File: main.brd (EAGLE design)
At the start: 78.8 x 63 mm, 8 parts, among them X1 FH12-40S-0.5SH

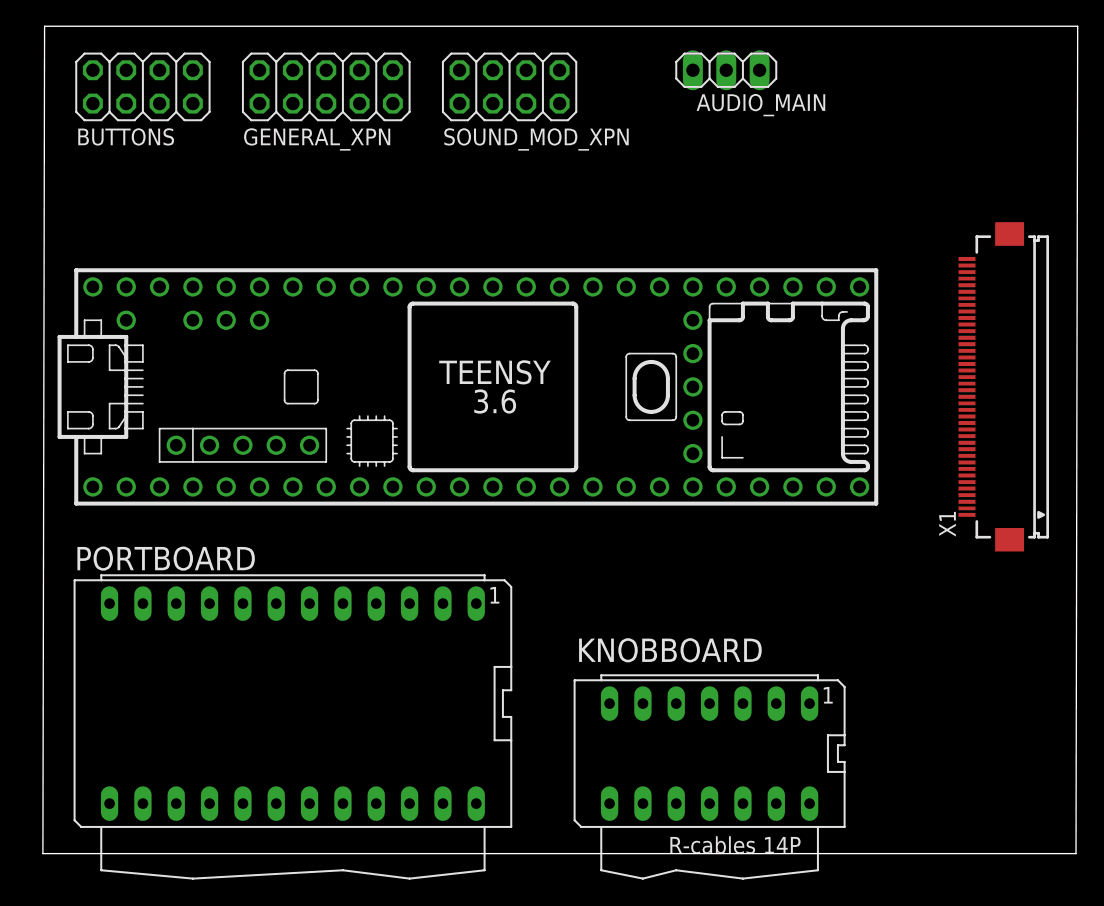
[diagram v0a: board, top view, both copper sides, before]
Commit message: Milestone fully drafted
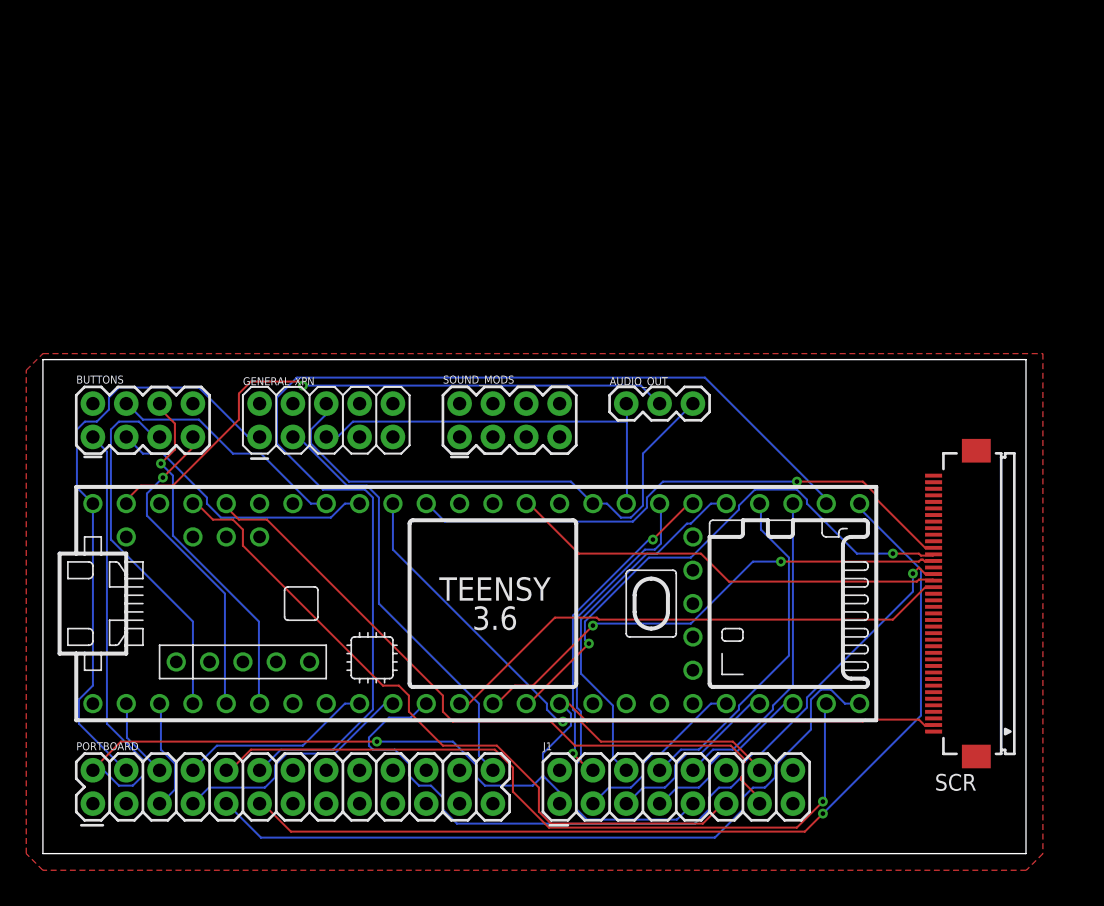
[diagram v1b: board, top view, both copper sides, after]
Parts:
- removed AUDIO_MAIN: (no value), pinhead:1X03
- removed KNOBBOARD: (no value), con-dil:IC14PL
- removed SOUND_MOD_XPN: (no value), pinhead:2X04
- removed X1: FH12-40S-0.5SH, con-hirose:FH12-40S-0.5SH
- added AUDIO_OUT: (no value), SparkFun-Connectors:1X03
- added J1: (no value), SparkFun-Connectors:2X8
- added SCR: FH12-40S-0.5SH, con-hirose:FH12-40S-0.5SH
- added SOUND_MODS: (no value), SparkFun-Connectors:2X4
- BUTTONS: device pinhead:2X04 -> SparkFun-Connectors:2X4
- GENERAL_XPN: device pinhead:2X05 -> SparkFun-Connectors:2X5
- PORTBOARD: device con-dil:IC24PL -> SparkFun-Connectors:2X13
- moved GENERAL_XPN 27.1 mm to (16.5, 31.8)
- moved BUTTONS 25.4 mm to (7.62, 33.0)
- moved PORTBOARD 17.0 mm to (3.81, 3.81), turned to 0 degrees
- moved U$1 16.5 mm to (31.8, 19.1)
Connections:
- removed net N$13: U$1.28
- removed net N$14: U$1.29
- removed net N$15: U$1.30
- removed net N$18: U$1.23/A9
- removed net N$19: U$1.22/A8
- removed net N$24: U$1.17/A3
- removed net N$30: U$1.35/A16
- removed net N$31: U$1.36/A17
- removed net N$32: U$1.37/A18
- removed net N$33: U$1.38/A19
- removed net N$34: U$1.39/A20
- new net USBDATA+: PORTBOARD.13
- new net USBDATA-: PORTBOARD.14
- net +12V: now also PORTBOARD.26
- net +3V3: now also J1.1, PORTBOARD.2, SCR.2; no longer KNOBBOARD.1, PORTBOARD.24, X1.2
- net +5V: now also PORTBOARD.4; no longer PORTBOARD.23
- net AUDIO_GND: now also AUDIO_OUT.2; no longer AUDIO_MAIN.2
- net AUDIO_L: now also AUDIO_OUT.1; no longer AUDIO_MAIN.1
- net AUDIO_R: now also AUDIO_OUT.3; no longer AUDIO_MAIN.3
- net GND: now also J1.2, PORTBOARD.3, SCR.1; no longer KNOBBOARD.14, PORTBOARD.2, X1.1
- net JOYSTICK_B: now also J1.14, U$1.17/A3; no longer KNOBBOARD.8
- net JOYSTICK_X: now also J1.11, U$1.23/A9; no longer KNOBBOARD.6
- net JOYSTICK_Y: now also J1.13, U$1.22/A8; no longer KNOBBOARD.7
- net MIDIIN1: now also PORTBOARD.6; no longer PORTBOARD.22
- net MIDIIN2: now also PORTBOARD.8; no longer PORTBOARD.21
- net MIDIIN3: now also PORTBOARD.10; no longer PORTBOARD.20
- net MIDIIN4: now also PORTBOARD.12; no longer PORTBOARD.19
- net MIDIOUT1: now also PORTBOARD.5; no longer PORTBOARD.3
- net MIDIOUT2: now also PORTBOARD.7; no longer PORTBOARD.4
- net MIDIOUT3: now also PORTBOARD.9; no longer PORTBOARD.5
- net MIDIOUT4: now also PORTBOARD.11; no longer PORTBOARD.6
- net ROTENC1_A: now also J1.3, U$1.28; no longer KNOBBOARD.2
- net ROTENC1_B: now also J1.5, U$1.29; no longer KNOBBOARD.3
- net ROTENC2_A: now also J1.7, U$1.30; no longer KNOBBOARD.4
- net ROTENC2_B: now also J1.9, U$1.39/A20; no longer KNOBBOARD.5
- net ROTENC3_A: now also J1.4, U$1.38/A19; no longer KNOBBOARD.13
- net ROTENC3_B: now also J1.6, U$1.37/A18; no longer KNOBBOARD.12
- net ROTENC4_A: now also J1.8, U$1.36/A17; no longer KNOBBOARD.11
- net ROTENC4_B: now also J1.10, U$1.35/A16; no longer KNOBBOARD.10
- net SCR_BL: now also SCR.29; no longer X1.29
- net SCR_CLK: now also SCR.24; no longer X1.24
- net SCR_CS: now also SCR.23; no longer X1.23
- net SCR_DC: now also SCR.25; no longer X1.25
- net SCR_MOSI: now also SCR.27; no longer X1.27
- net SCR_MOSO: now also SCR.28; no longer X1.28
- net SDCLK: now also PORTBOARD.19; no longer PORTBOARD.9
- net SDCMD: now also PORTBOARD.20; no longer PORTBOARD.16
- net SDDATA0: now also PORTBOARD.15; no longer PORTBOARD.7
- net SDDATA1: now also PORTBOARD.16; no longer PORTBOARD.18
- net SDDATA2: now also PORTBOARD.17; no longer PORTBOARD.8
- net SDDATA3: now also PORTBOARD.18; no longer PORTBOARD.17
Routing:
- net +3V3: track 0.00 -> 108.3 mm, vias 0 -> 1
- net MIDIIN4: track 0.00 -> 86.0 mm
- net MIDIOUT4: track 0.00 -> 73.1 mm, vias 0 -> 1
- net SCR_DC: track 0.00 -> 63.2 mm, vias 0 -> 1
- net MIDIIN3: track 0.00 -> 58.1 mm, vias 0 -> 1
- net MIDIOUT3: track 0.00 -> 56.9 mm
- net JOYSTICK_X: track 0.00 -> 53.9 mm
- net JOYSTICK_Y: track 0.00 -> 52.6 mm
- net AUDIO_GND: track 0.00 -> 46.5 mm, vias 0 -> 1
- net +5V: track 0.00 -> 45.8 mm
- net SCR_BL: track 0.00 -> 43.2 mm, vias 0 -> 1
- net SCR_MOSO: track 0.00 -> 41.7 mm, vias 0 -> 2
- net AUDIO_R: track 0.00 -> 41.0 mm
- net SCR_CS: track 0.00 -> 39.9 mm
- net JOYSTICK_B: track 0.00 -> 38.9 mm, vias 0 -> 1
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- added copper zone on layer 1, net GND
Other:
- board size 78.8 x 63 mm -> 74.9 x 37.6 mm
